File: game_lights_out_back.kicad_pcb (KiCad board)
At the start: 2 copper layers, 171 x 127.3 mm, 5 parts

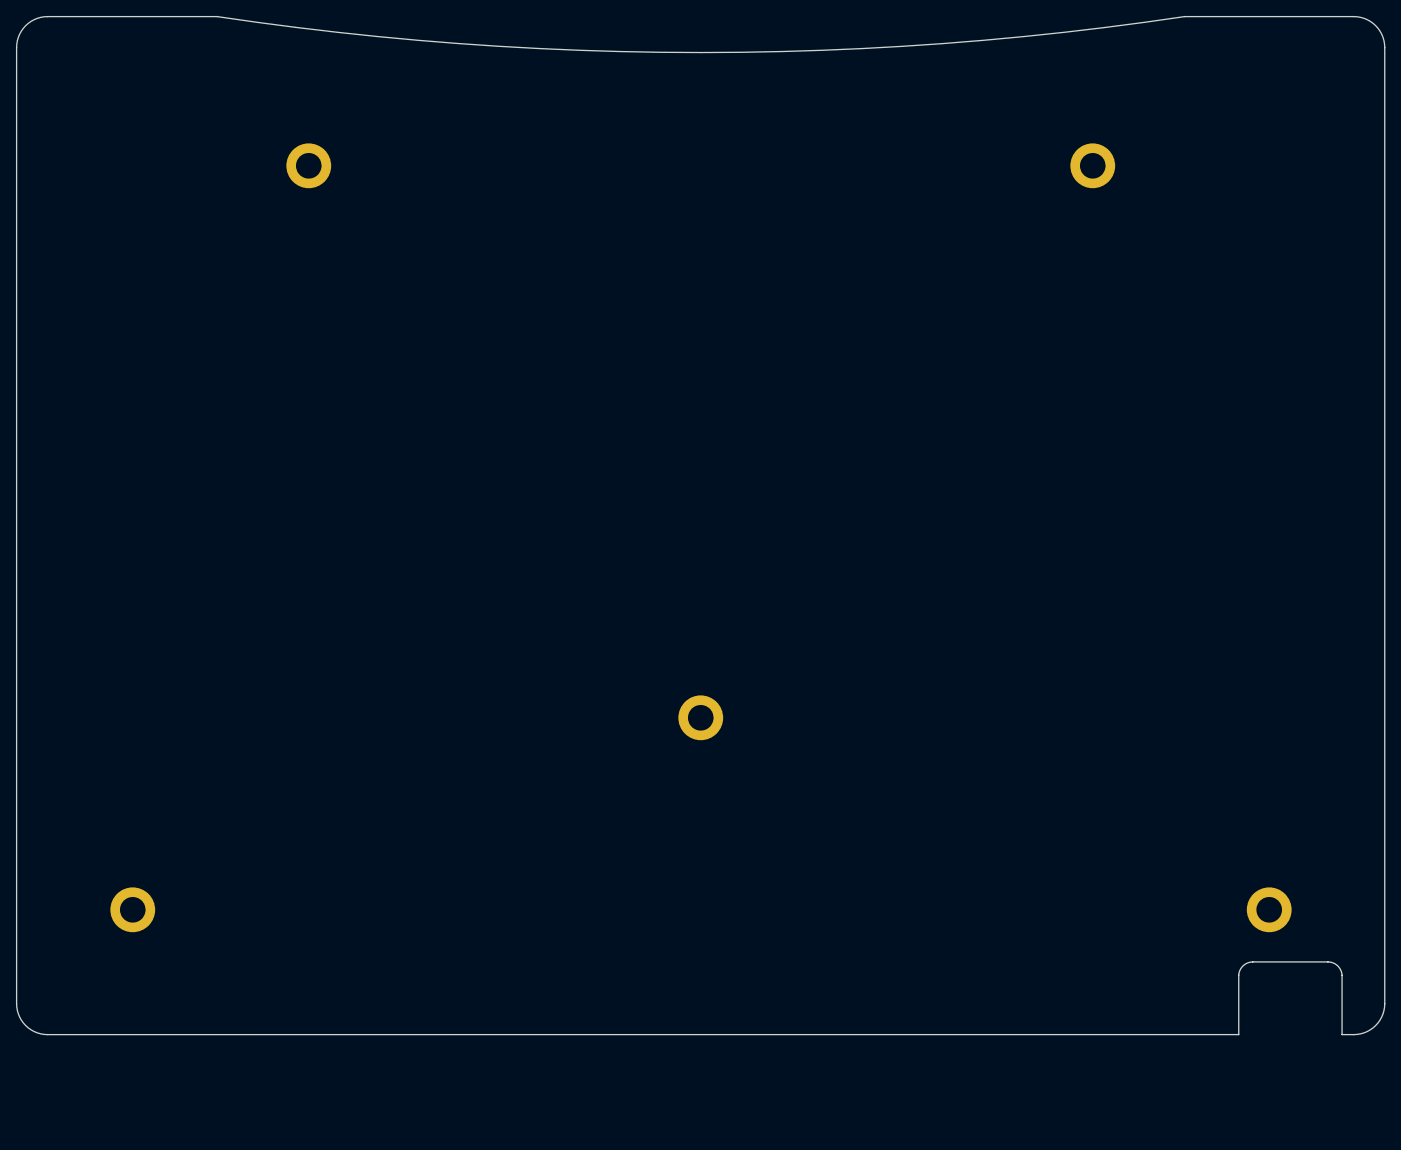
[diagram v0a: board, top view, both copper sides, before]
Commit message: Finilized decorations
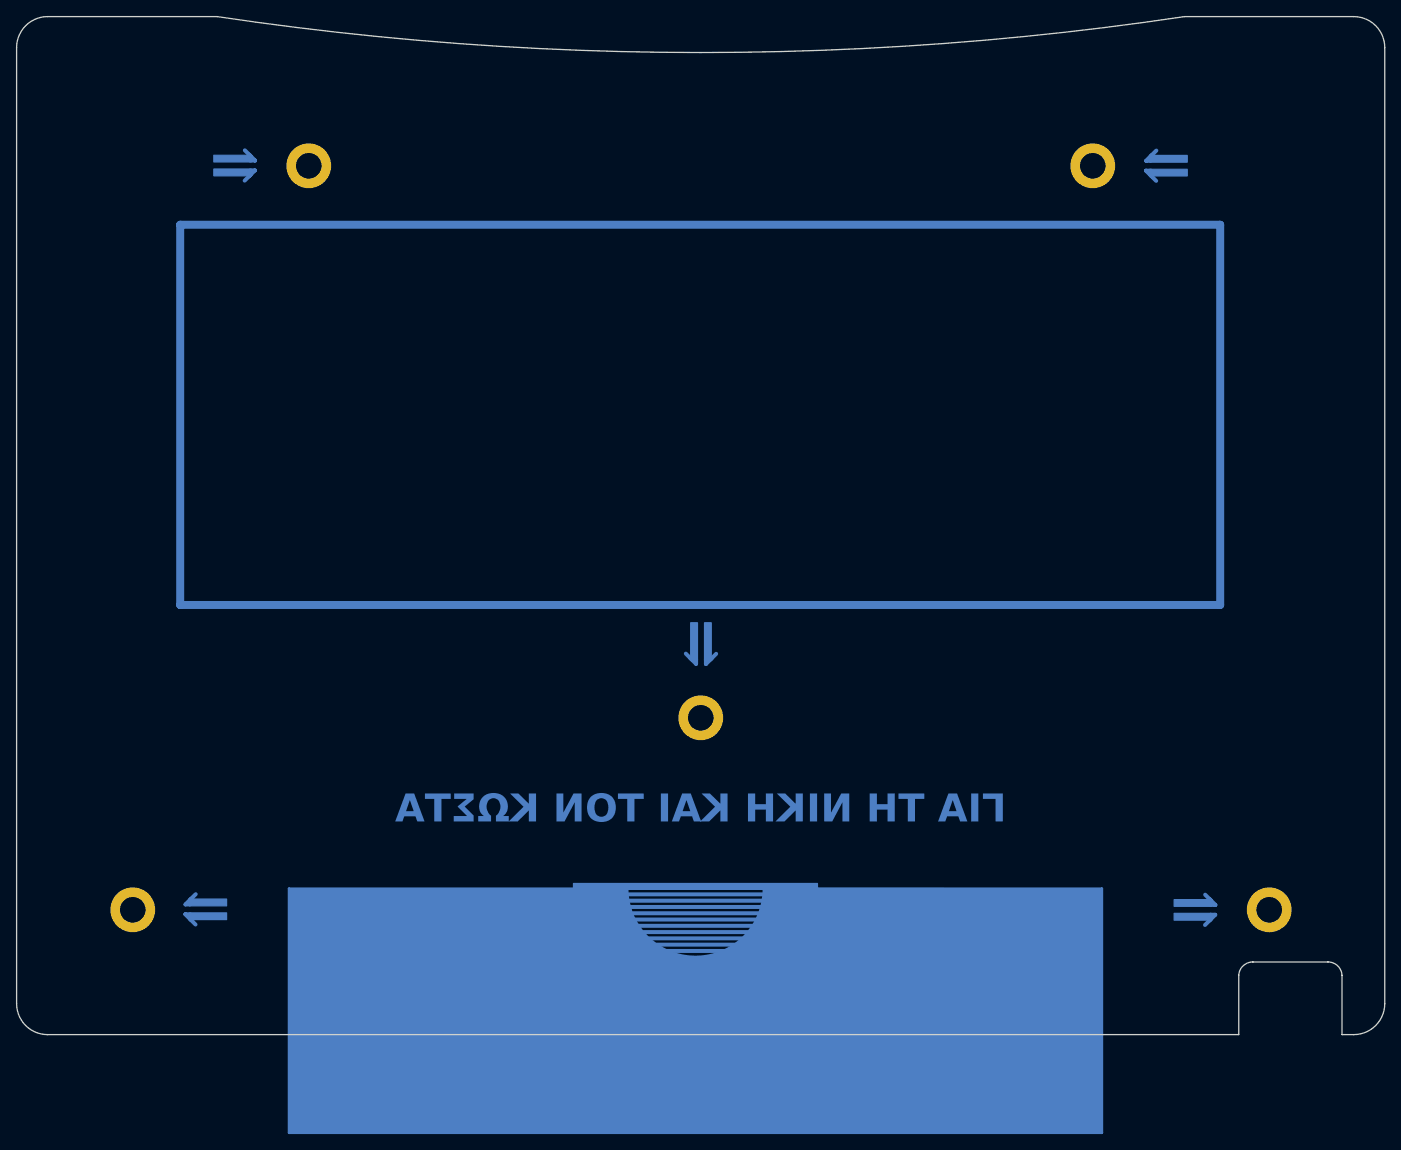
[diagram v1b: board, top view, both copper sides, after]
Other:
- board text added: "ΓΙΑ ΤΗ ΝΙΚΗ ΚΑΙ ΤΟΝ ΚΩΣΤΑ"
